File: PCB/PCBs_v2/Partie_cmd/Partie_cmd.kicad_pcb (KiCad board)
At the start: 4 copper layers, 79.2 x 75 mm, 74 parts, among them J1 Barrel_Jack, J10 Conn_01x02, J2 Conn_01x04_Socket, J3 Conn_01x04_Socket, J4 Conn_01x12, J6 Conn_01x04, J7 Conn_01x04, J9 Conn_01x02, U1 ESP32-S3-DEVKITC-1-N8R2, U2 BU18SD5WG-TL, U3 BU33SD5WG-TR, U4 XL1509-5.0

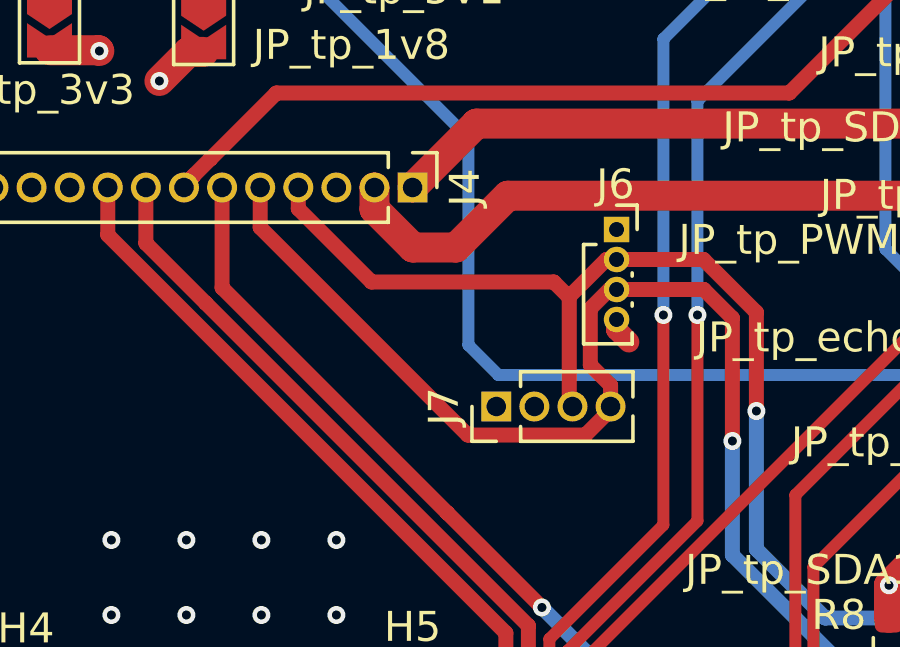
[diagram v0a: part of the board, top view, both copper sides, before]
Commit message: Fin routage 1.2
pour de vrai cette foix?
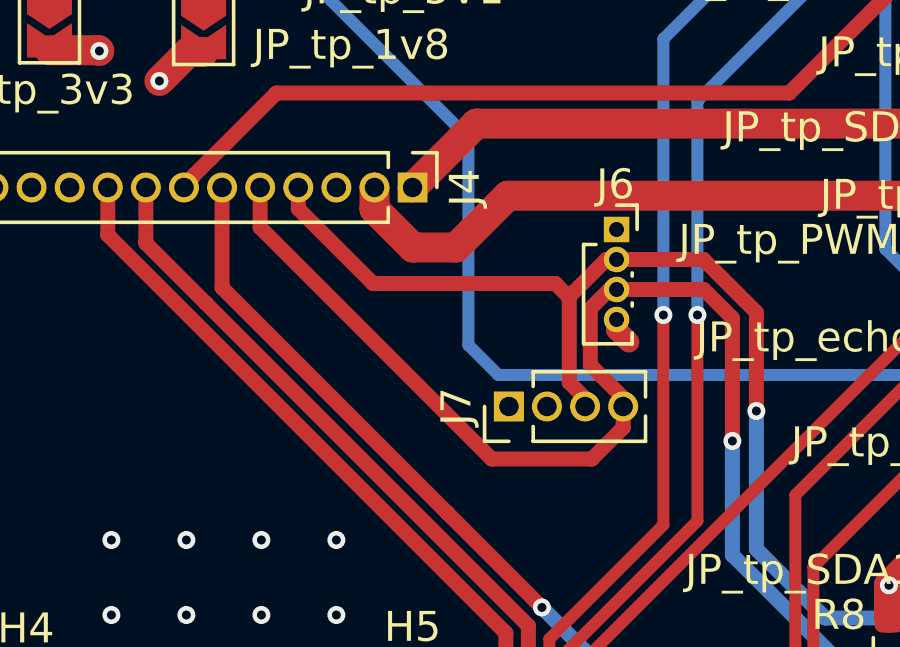
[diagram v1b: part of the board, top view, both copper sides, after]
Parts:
- moved J7 0.42 mm to (133.2, 88.0)
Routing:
- net 5V: track 242.9 -> 240.6 mm
- net SCL: track 48.6 -> 50.2 mm
